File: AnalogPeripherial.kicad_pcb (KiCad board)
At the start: 2 copper layers, 52 parts, among them J1 USART, J2 SWD, J3 USB_B_Mini, SW1 record, SW2 replay, SW3 SW_Nidec_CAS-120A1, U1 LD1117S33TR_SOT223, U2 STM32F373CCTx, U3 LM386, U5 TLV9061xDBV, Y1 Crystal

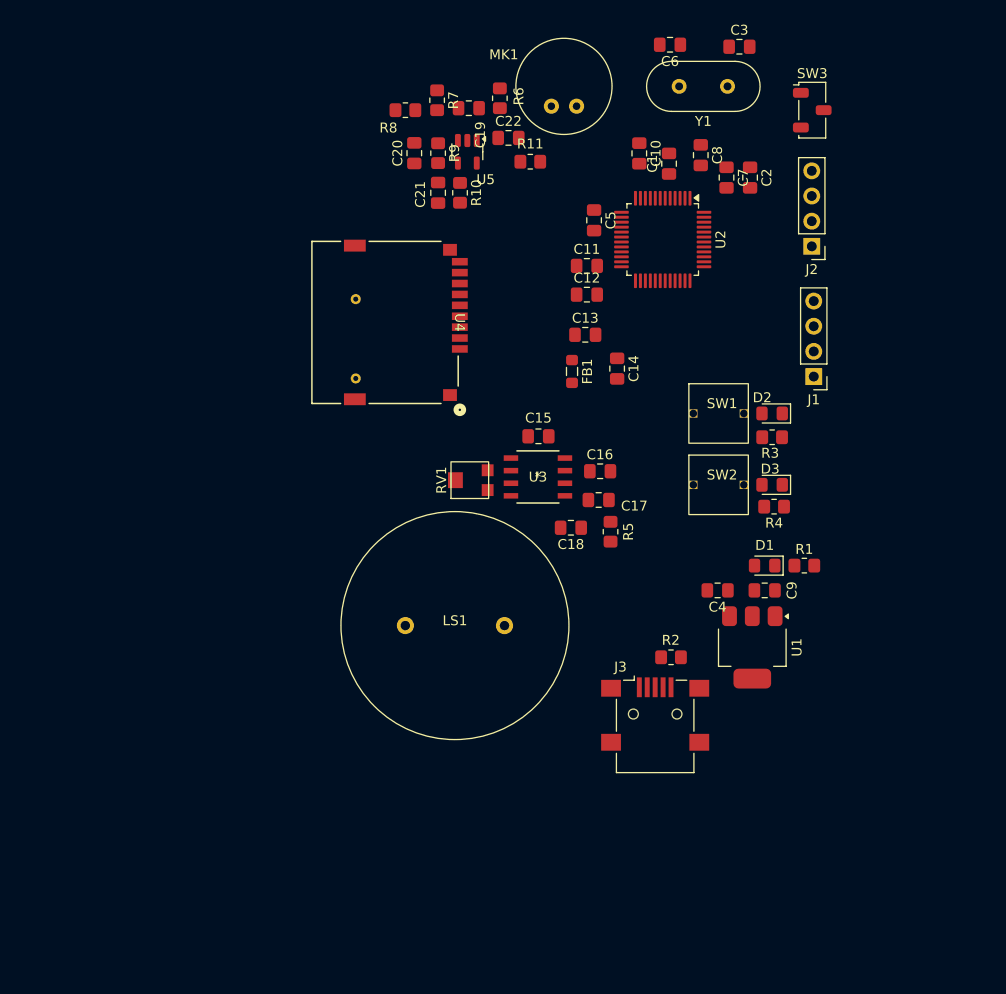
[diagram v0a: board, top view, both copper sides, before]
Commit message: PCB design still in progress
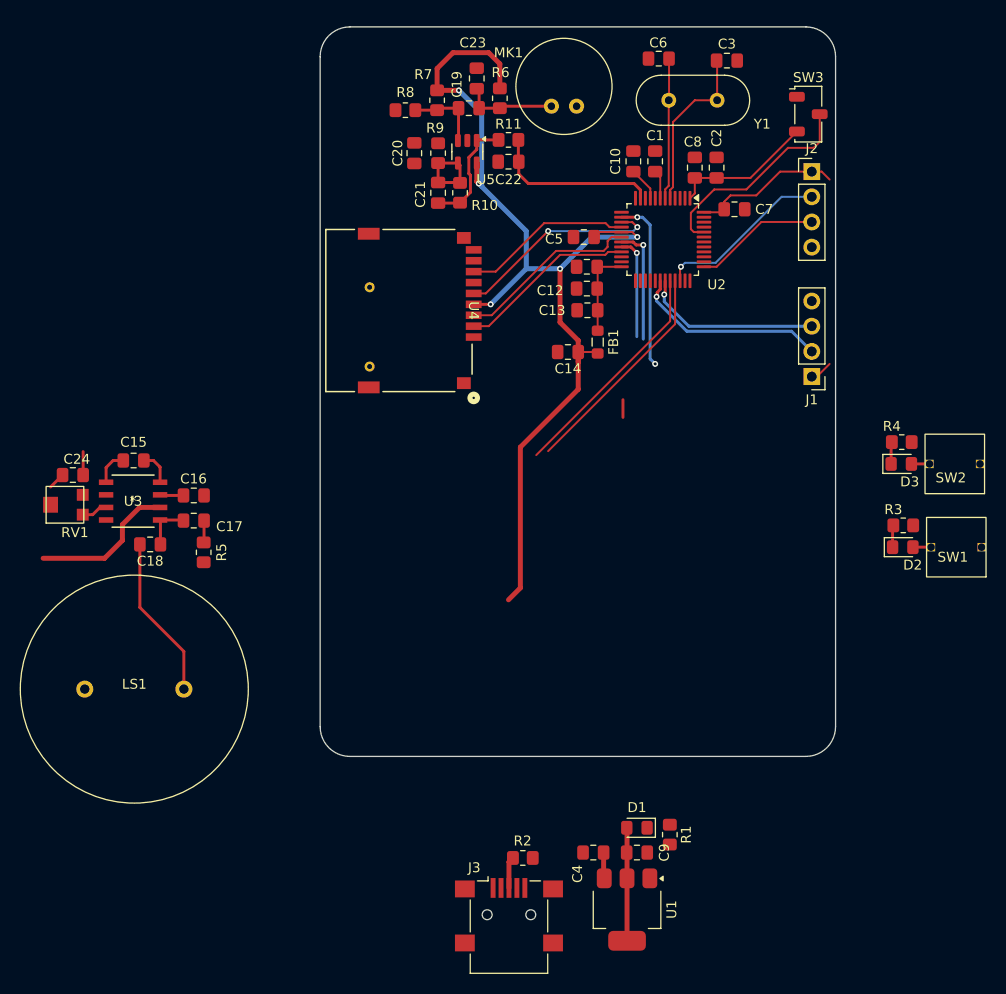
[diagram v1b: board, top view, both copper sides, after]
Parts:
- added C23: 33p, Capacitor_SMD:C_0805_2012Metric_Pad1.18x1.45mm_HandSolder, F.Cu at (124.0, 70.0)
- added C24: 10u, Capacitor_SMD:C_0805_2012Metric_Pad1.18x1.45mm_HandSolder, F.Cu at (83.2, 110.0)
- C16: value 100p -> 100u
- C17: value 0.047u -> 0.05u
- C18: value 470u -> 250u
- C19: value 330n -> 68n
- C20: value 47u -> 40u
- C21: value 120p -> 995p
- C22: value 3.3u -> 150n
- R11: value 10k -> 100
- R6: value 5.9k -> 2.2k
- R7, R8: value 200k -> 100k
- R9: value 787 -> 78.7
- moved C18 42.5 mm to (91.0, 117.0)
- moved R5 41.1 mm to (96.5, 117.8)
- moved C16 41.1 mm to (95.5, 112.1)
- moved RV1 40.9 mm to (82.5, 113.0)
- moved C15 40.9 mm to (89.4, 108.5)
- moved U3 40.9 mm to (89.3, 112.6)
- moved C17 40.9 mm to (95.5, 114.6)
- moved LS1 33.0 mm to (89.5, 131.6)
- moved R1 30.3 mm to (143.5, 146.3), turned to -90 degrees
- moved C9 29.4 mm to (140.2, 148.1)
- moved D1 29.4 mm to (140.2, 145.6)
- moved U1 29.3 mm to (139.2, 153.8)
- moved C4 29.3 mm to (135.8, 148.1)
- moved SW1 27.5 mm to (172.4, 117.3), turned to 180 degrees
- moved R2 25.2 mm to (128.7, 148.6)
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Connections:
- net /NRST renamed Net-(U2-NRST)
- C22 pad 1: Net-(C21-Pad2) -> GND
- R11 pad 1: GND -> ADC1_IN1
- R11 pad 2: ADC1_IN1 -> Net-(C21-Pad2)
- RV1 pad 1: DAC1_OUT1 -> Net-(C24-Pad2)
- U2 pad 1: GND -> 3V3
- U2 pad 17: GND -> 3V3
- U2 pad 21: unconnected-(U2-PE8-Pad21) -> SPI1_NSS
- U2 pad 24: GND -> 3VA3
- U2 pad 38: SPI1_NSS -> unconnected-(U2-PA15-Pad38)
- U2 pad 48: GND -> 3V3
- U2 pad 9: GND -> 3VA3
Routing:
- net 3V3: track 0.00 -> 145.5 mm, vias 0 -> 5
- net USB+: track 0.00 -> 25.7 mm
- net USB-: track 0.00 -> 23.2 mm
- net BOOT0: track 0.00 -> 21.9 mm
- net SPI1_SCK: track 0.00 -> 21.1 mm, vias 0 -> 2
- net USART1_TX: track 0.00 -> 20.0 mm, vias 0 -> 1
- net DAC1_OUT1: track 0.00 -> 19.9 mm, vias 0 -> 2
- net SPI1_MOSI: track 0.00 -> 18.5 mm
- net USART1_RX: track 0.00 -> 18.1 mm, vias 0 -> 1
- net SPI1_NSS: track 0.00 -> 18.0 mm
- net SWDIO: track 0.00 -> 17.6 mm, vias 0 -> 1
- net VBUS: track 0.00 -> 17.5 mm
- net ADC1_IN1: track 0.00 -> 17.2 mm
- net HSE_IN: track 0.00 -> 17.2 mm
- net SPI1_MISO: track 0.00 -> 17.1 mm
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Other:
- board outline added: 52 x 73.6 mm
